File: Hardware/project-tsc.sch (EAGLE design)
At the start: 105 parts, among them IC1 BQ25180YBGR, IC2 DRV2605YZFR, IC3 BMA421, IC9 RT6160AWSC, J1 TC2030-IDC_TC2030-IDC, J2 503480-2400_503480-2400, J4 KH-TYPE-C-16P, Q1 20V/4.2A/52mΩ/1.4W, Q3 SI1308EDL-T1-GE3, U1 NRF52840_QF, U2 ESP32_C6_LIBRARY_MAX17048G+T10, X1 32MHz, X2 32.726kHz

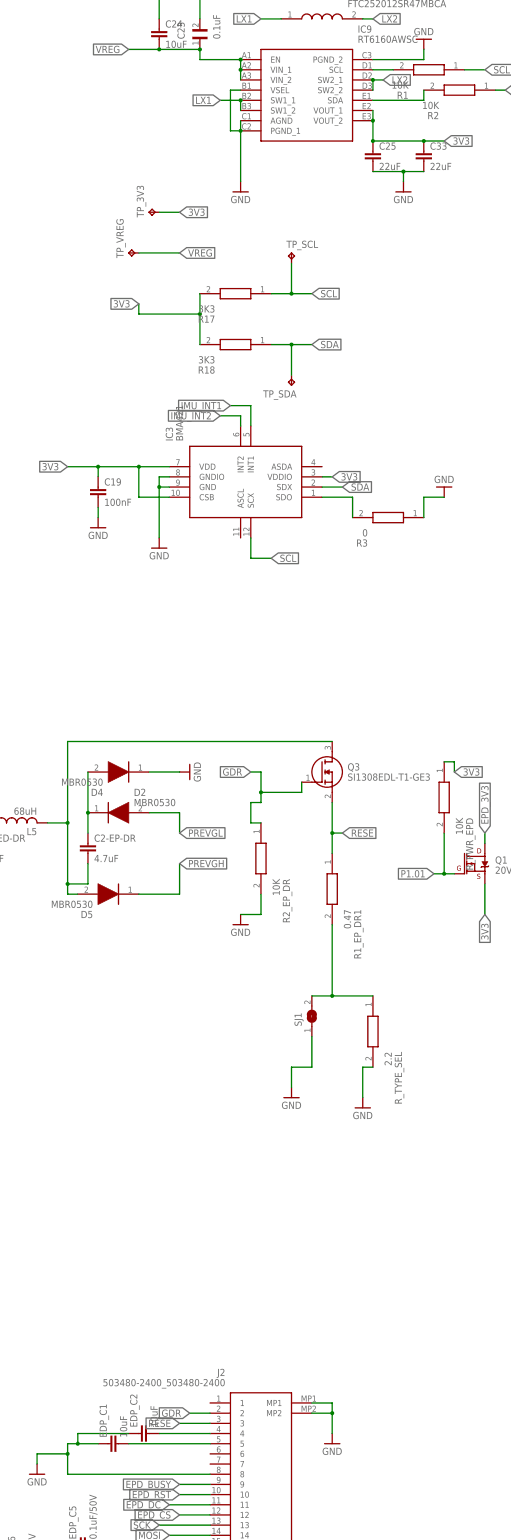
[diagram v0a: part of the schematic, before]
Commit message: Refactor code structure for improved readability and maintainability
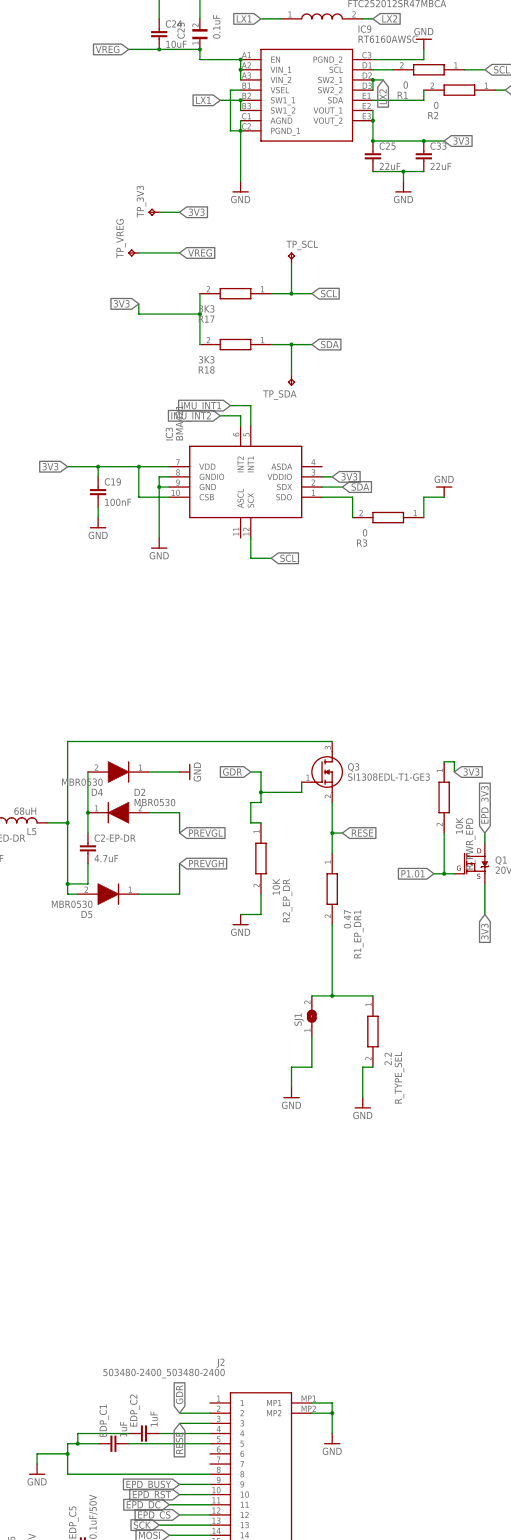
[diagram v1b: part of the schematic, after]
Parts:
- EDP_C1, EDP_C2: value 10uF -> 1uF
- R1, R2: value 10K -> 0
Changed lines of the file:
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@@
 <part name="SUPPLY11" library="InkTime_v5" library_urn="urn:adsk.wipprod:fs.file:vf.kHyW2j0lSQGBfLdbHOMXug" deviceset="POWER_SYMBOLS_GND-BAR" device="" value="GND"/>
 <part name="SUPPLY12" library="InkTime_v5" library_urn="urn:adsk.wipprod:fs.file:vf.kHyW2j0lSQGBfLdbHOMXug" deviceset="POWER_SYMBOLS_GND-BAR" device="" value="GND"/>
-<part name="R1" library="InkTime_v5" library_urn="urn:adsk.wipprod:fs.file:vf.kHyW2j0lSQGBfLdbHOMXug" deviceset="CPF0201D7K68C1_CPF0201D7K68C1" device="" value="10K"/>
-<part name="R2" library="InkTime_v5" library_urn="urn:adsk.wipprod:fs.file:vf.kHyW2j0lSQGBfLdbHOMXug" deviceset="CPF0201D7K68C1_CPF0201D7K68C1" device="" value="10K"/>
+<part name="R1" library="InkTime_v5" library_urn="urn:adsk.wipprod:fs.file:vf.kHyW2j0lSQGBfLdbHOMXug" deviceset="CPF0201D7K68C1_CPF0201D7K68C1" device="" value="0"/>
+<part name="R2" library="InkTime_v5" library_urn="urn:adsk.wipprod:fs.file:vf.kHyW2j0lSQGBfLdbHOMXug" deviceset="CPF0201D7K68C1_CPF0201D7K68C1" device="" value="0"/>
 <part name="C25" library="InkTime_v5" library_urn="urn:adsk.wipprod:fs.file:vf.kHyW2j0lSQGBfLdbHOMXug" deviceset="NORDIC_NRF_3_CAPACITOR" device="_0201_L" value="22uF"/>
 <part name="C33" library="InkTime_v5" library_urn="urn:adsk.wipprod:fs.file:vf.kHyW2j0lSQGBfLdbHOMXug" deviceset="NORDIC_NRF_3_CAPACITOR" device="_0201_L" value="22uF"/>
@@
 <part name="C27" library="InkTime_v5" library_urn="urn:adsk.wipprod:fs.file:vf.kHyW2j0lSQGBfLdbHOMXug" deviceset="GRM011R60J152KE01L_2_GRM011R60J152KE01L" device="" value="0.1uF"/>
 <part name="J2" library="InkTime_v5" library_urn="urn:adsk.wipprod:fs.file:vf.kHyW2j0lSQGBfLdbHOMXug" deviceset="503480-2400_503480-2400" device=""/>
-<part name="EDP_C2" library="InkTime_v5" library_urn="urn:adsk.wipprod:fs.file:vf.kHyW2j0lSQGBfLdbHOMXug" deviceset="NORDIC_NRF_3_CAPACITOR" device="_0201_L" value="10uF"/>
-<part name="EDP_C1" library="InkTime_v5" library_urn="urn:adsk.wipprod:fs.file:vf.kHyW2j0lSQGBfLdbHOMXug" deviceset="NORDIC_NRF_3_CAPACITOR" device="_0201_L" value="10uF"/>
+<part name="EDP_C2" library="InkTime_v5" library_urn="urn:adsk.wipprod:fs.file:vf.kHyW2j0lSQGBfLdbHOMXug" deviceset="NORDIC_NRF_3_CAPACITOR" device="_0201_L" value="1uF"/>
+<part name="EDP_C1" library="InkTime_v5" library_urn="urn:adsk.wipprod:fs.file:vf.kHyW2j0lSQGBfLdbHOMXug" deviceset="NORDIC_NRF_3_CAPACITOR" device="_0201_L" value="1uF"/>
 <part name="EDP_C5" library="InkTime_v5" library_urn="urn:adsk.wipprod:fs.file:vf.kHyW2j0lSQGBfLdbHOMXug" deviceset="NORDIC_NRF_3_CAPACITOR" device="_0201_L" value="0.1uF/50V"/>
 <part name="EDP_C6" library="InkTime_v5" library_urn="urn:adsk.wipprod:fs.file:vf.kHyW2j0lSQGBfLdbHOMXug" deviceset="NORDIC_NRF_3_CAPACITOR" device="_0201_L" value="1uF/50V"/>
@@
 </instance>
 <instance part="J2" gate="G$1" x="-73.66" y="-358.14" smashed="yes" rot="MR0">
-<attribute name="NAME" x="-95.25" y="-350.52" size="1.778" layer="95" rot="MR0" align="center-left"/>
-<attribute name="VALUE" x="-95.25" y="-353.06" size="1.778" layer="96" rot="MR0" align="center-left"/>
+<attribute name="NAME" x="-95.25" y="-347.98" size="1.778" layer="95" rot="MR0" align="center-left"/>
+<attribute name="VALUE" x="-95.25" y="-350.52" size="1.778" layer="96" rot="MR0" align="center-left"/>
 </instance>
 <instance part="EDP_C2" gate="C$1" x="-116.84" y="-365.76" smashed="yes" rot="R90">
@@
 <wire x1="-58.42" y1="-27.94" x2="-55.88" y2="-27.94" width="0.1524" layer="91"/>
 <junction x="-58.42" y="-27.94"/>
-<label x="-55.88" y="-27.94" size="1.778" layer="95" xref="yes"/>
+<label x="-55.88" y="-27.94" size="1.778" layer="95" rot="R270" xref="yes"/>
 </segment>
 </net>
@@
 </segment>
 <segment>
-<wire x1="-104.14" y1="-360.68" x2="-99.06" y2="-360.68" width="0.1524" layer="91"/>
+<wire x1="-106.68" y1="-360.68" x2="-99.06" y2="-360.68" width="0.1524" layer="91"/>
 <pinref part="J2" gate="G$1" pin="2"/>
-<label x="-104.14" y="-360.68" size="1.778" layer="95" rot="R180" xref="yes"/>
+<label x="-106.68" y="-360.68" size="1.778" layer="95" rot="R90" xref="yes"/>
 </segment>
 </net>
@@
 <wire x1="-106.68" y1="-363.22" x2="-99.06" y2="-363.22" width="0.1524" layer="91"/>
 <pinref part="J2" gate="G$1" pin="3"/>
-<label x="-106.68" y="-363.22" size="1.778" layer="95" rot="R180" xref="yes"/>
+<label x="-106.68" y="-363.22" size="1.778" layer="95" rot="R270" xref="yes"/>
 </segment>
 </net>
@@
 </sheet>
 </sheets>
+<errors>
+</errors>
 </schematic>
 </drawing>
